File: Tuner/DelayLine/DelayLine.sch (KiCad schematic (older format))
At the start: 85 parts, among them J1 Conn_Coaxial, J10 Conn_Coaxial, J11 Conn_Coaxial, J12 Conn_Coaxial, J13 Conn_01x01, J14 Conn_01x01, J15 Conn_01x01, J16 Conn_01x01, J17 Conn_02x10_Odd_Even, J18 Conn_Coaxial, J19 Conn_Coaxial, J20 Conn_Coaxial, J21 Conn_Coaxial, J22 Conn_Coaxial, J23 Conn_Coaxial, J24 Conn_01x01, J25 Conn_01x01, J26 Conn_01x01, J27 Conn_01x01, J28 Conn_01x01, J29 Conn_Coaxial, J3 Conn_Coaxial, J31 Conn_Coaxial, J32 Conn_01x01, J33 Conn_01x01, J34 Conn_01x01, J35 Conn_01x01, J5 Conn_Coaxial, J6 Conn_Coaxial, J7 Conn_Coaxial, J8 Conn_01x02, J9 Conn_01x02

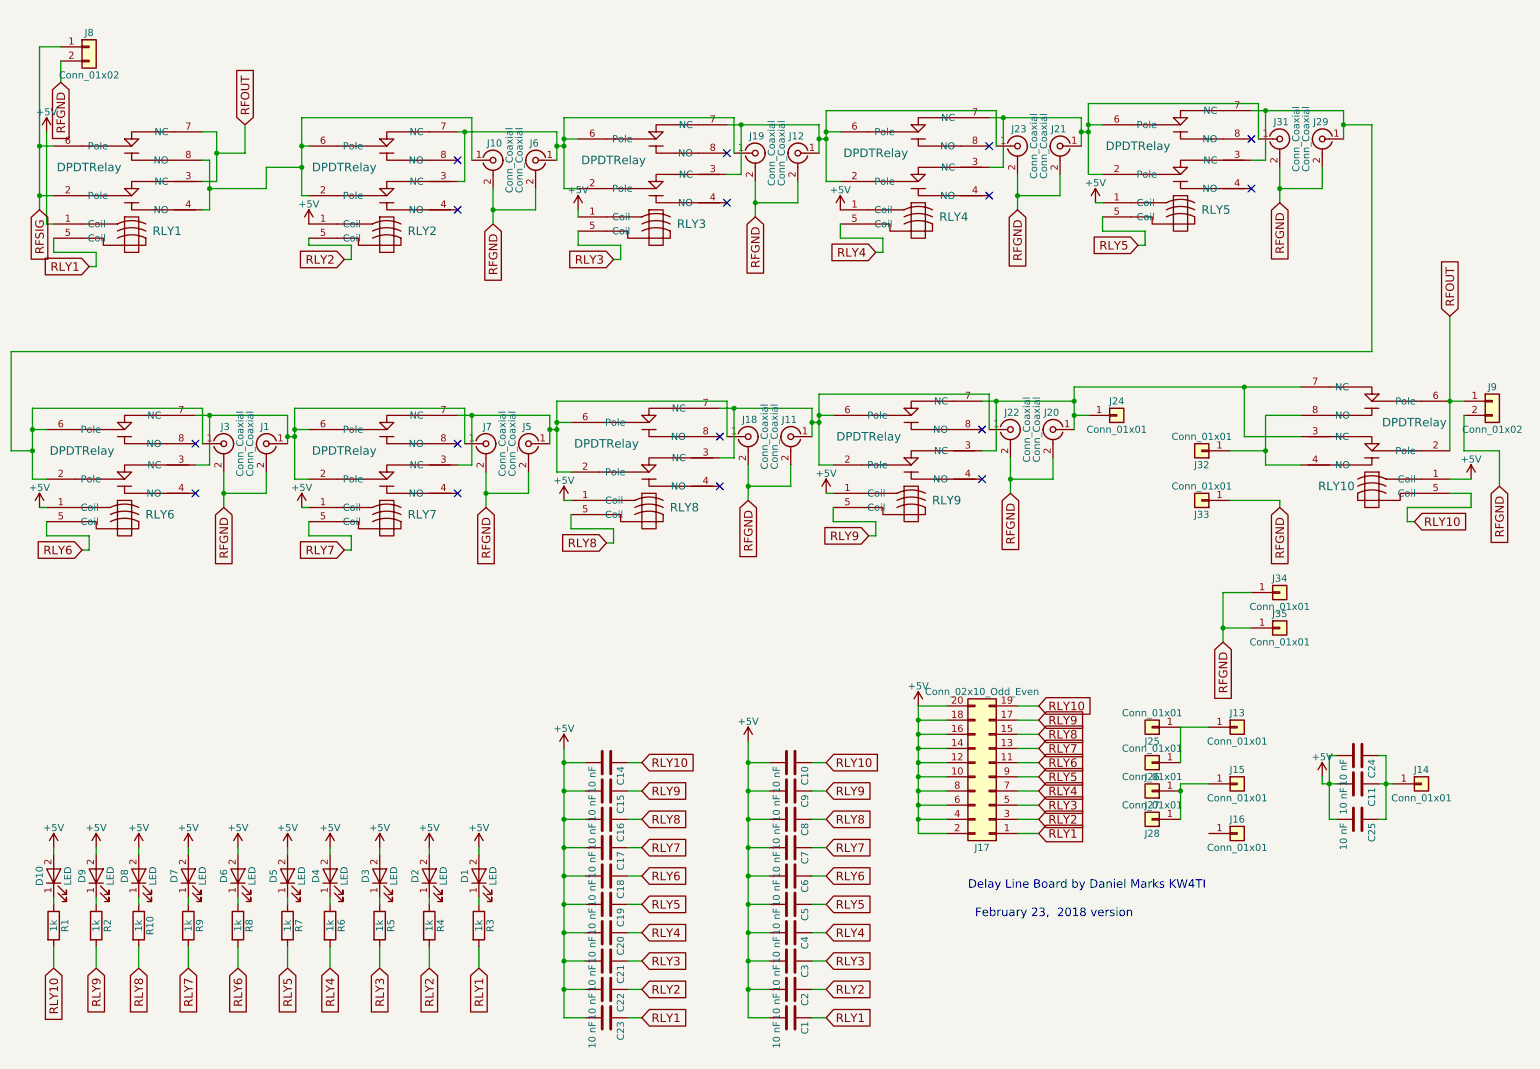
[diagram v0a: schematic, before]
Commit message: Stupid mistake, went to another method
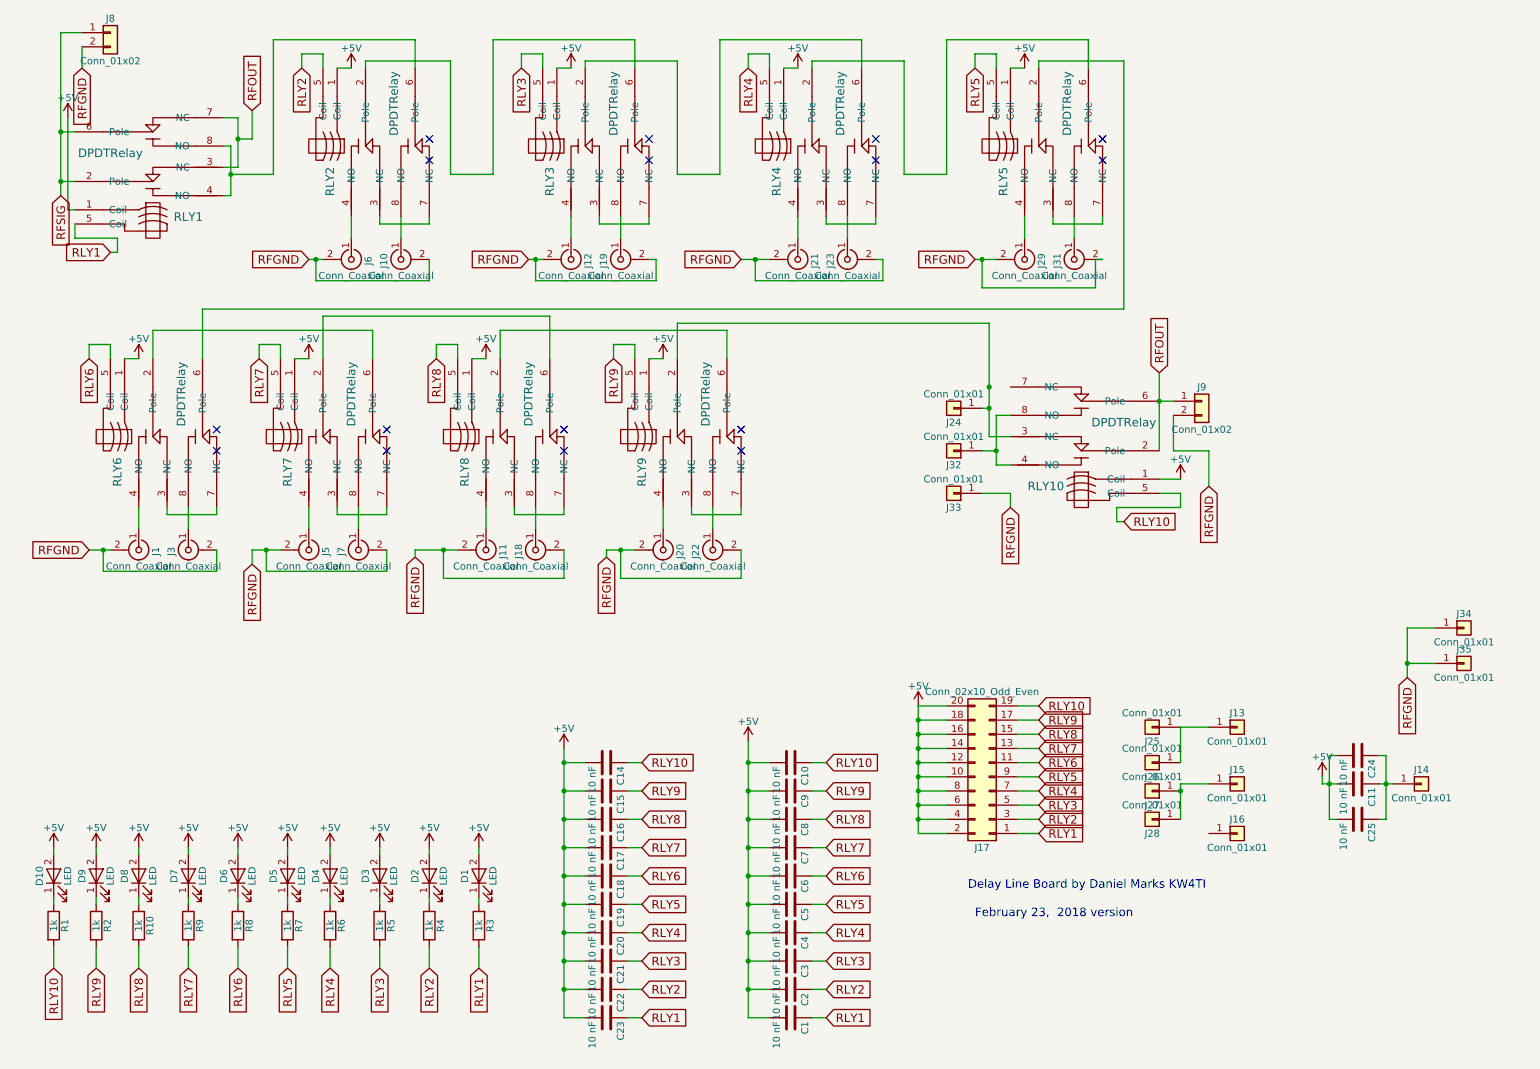
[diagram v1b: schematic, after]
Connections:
- net at RLY1.4 (NO), RLY1.8 (NO), RLY2.6 (Pole): no longer J10.1 (In), RLY2.2 (Pole)
- net at RLY2.4 (NO): now also J6.1 (In)
- net at RLY2.8 (NO): now also J10.1 (In)
- net at RLY3.4 (NO): now also J12.1 (In)
- net at RLY3.8 (NO): now also J19.1 (In)
- net at RLY4.4 (NO): now also J21.1 (In)
- net at RLY4.8 (NO): now also J23.1 (In)
- net at RLY5.4 (NO): now also J29.1 (In)
- net at RLY5.8 (NO): now also J31.1 (In)
- net at RLY6.4 (NO): now also J1.1 (In)
- net at RLY6.8 (NO): now also J3.1 (In)
- net at RLY7.4 (NO): now also J5.1 (In)
- net at RLY7.8 (NO): now also J7.1 (In)
- net at RLY8.4 (NO): now also J11.1 (In)
- net at RLY8.8 (NO): now also J18.1 (In)
- net at RLY9.4 (NO): now also J20.1 (In)
- net at RLY9.8 (NO): now also J22.1 (In)
- new net: J24.1 (Pin_1), RLY10.3 (NC), RLY9.2 (Pole)
- new net: RLY2.2 (Pole), RLY3.6 (Pole)
- new net: RLY2.3 (NC), RLY2.7 (NC)
- new net: RLY3.2 (Pole), RLY4.6 (Pole)
- new net: RLY3.3 (NC), RLY3.7 (NC)
- new net: RLY4.2 (Pole), RLY5.6 (Pole)
- new net: RLY4.3 (NC), RLY4.7 (NC)
- new net: RLY5.2 (Pole), RLY6.6 (Pole)
- new net: RLY5.3 (NC), RLY5.7 (NC)
- new net: RLY6.2 (Pole), RLY7.6 (Pole)
- new net: RLY6.3 (NC), RLY6.7 (NC)
- new net: RLY7.2 (Pole), RLY8.6 (Pole)
- new net: RLY7.3 (NC), RLY7.7 (NC)
- new net: RLY8.2 (Pole), RLY9.6 (Pole)
- new net: RLY8.3 (NC), RLY8.7 (NC)
- new net: RLY9.3 (NC), RLY9.7 (NC)
- now unconnected: RLY10.7 (NC)
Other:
- moved on the sheet: J10, J24, J32, J33, J34, J35, J6, J8, J9, RLY1, RLY10, RLY2
